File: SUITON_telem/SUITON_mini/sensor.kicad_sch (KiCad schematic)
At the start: 17 parts, among them U10 LSM6DSV320XTR, U6 MMC5983MA, U7 ISM330DHCXTR, U8 SAM-M10Q-00B, U9 BMP581

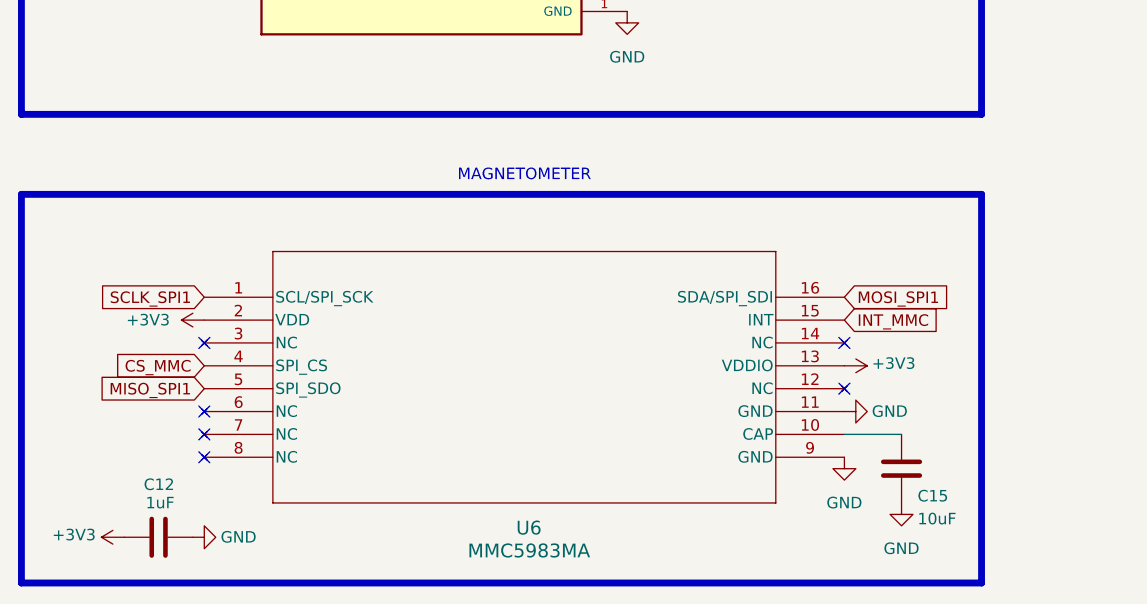
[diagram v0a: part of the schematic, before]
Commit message: New rf module
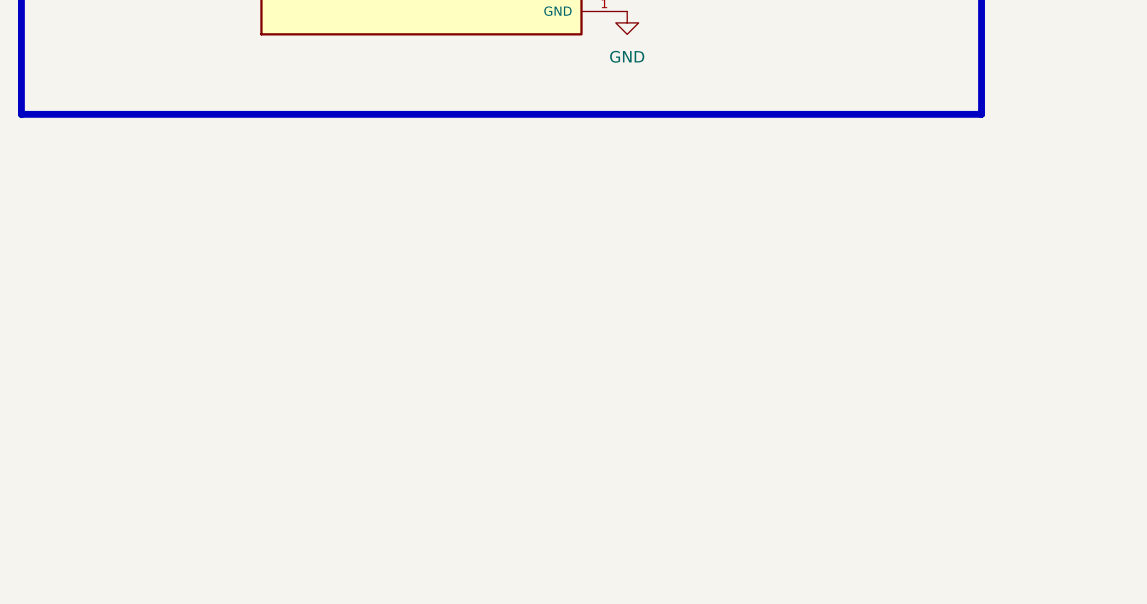
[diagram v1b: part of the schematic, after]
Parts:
- removed C12: 1uF, Capacitor_SMD:C_0603_1608Metric, symbol Device:C
- removed C15: 10uF, Capacitor_SMD:C_0603_1608Metric, symbol Device:C
- removed U6: MMC5983MA, MMC5983MA_MEM, symbol 2026-09-30_16-50-22:MMC5983MA
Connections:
- no-connect marks 11 -> 5
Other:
- note removed: "MAGNETOMETER"
